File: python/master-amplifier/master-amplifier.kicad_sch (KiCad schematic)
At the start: 8 parts, among them Q1 NPN

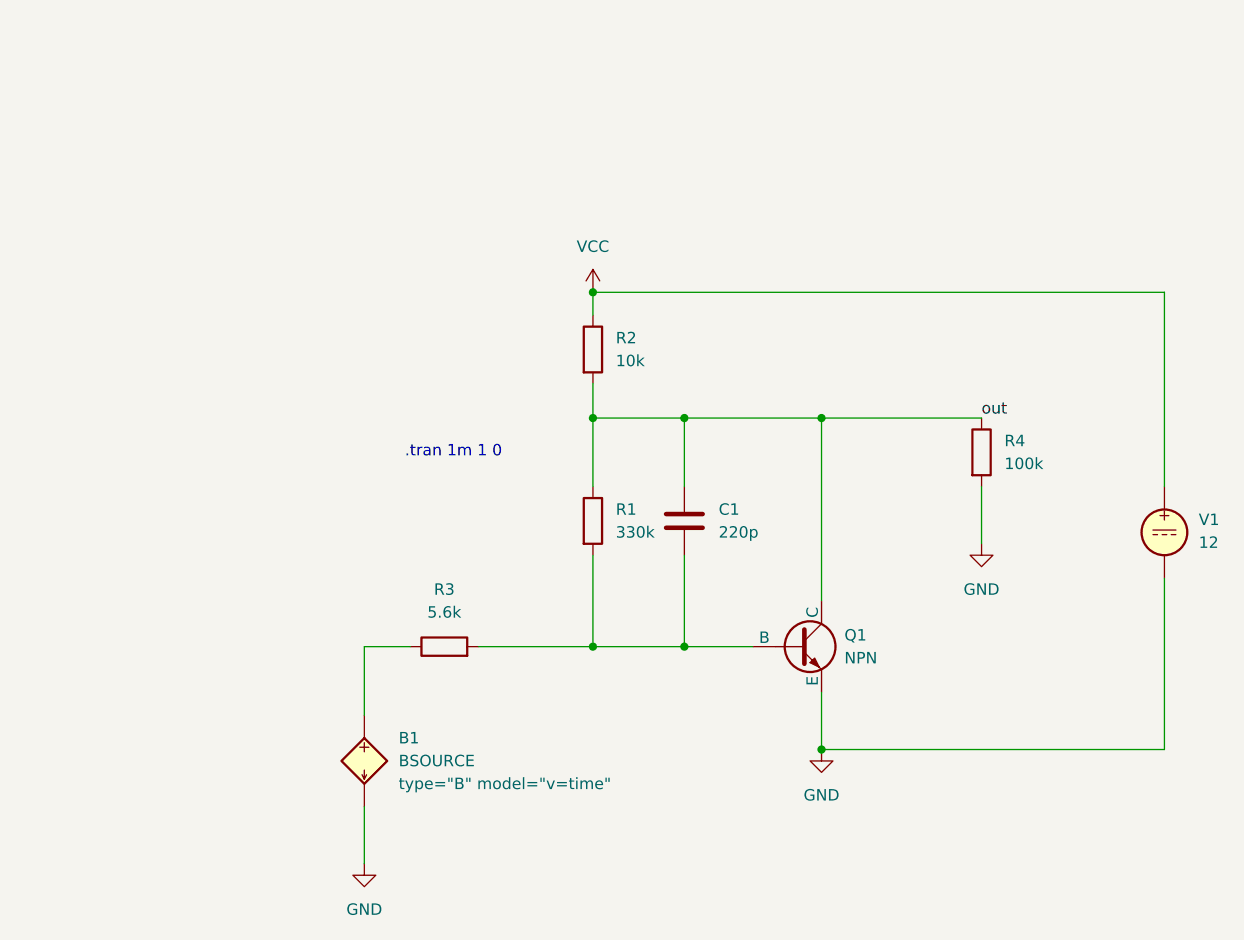
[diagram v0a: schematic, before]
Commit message: something in schematics
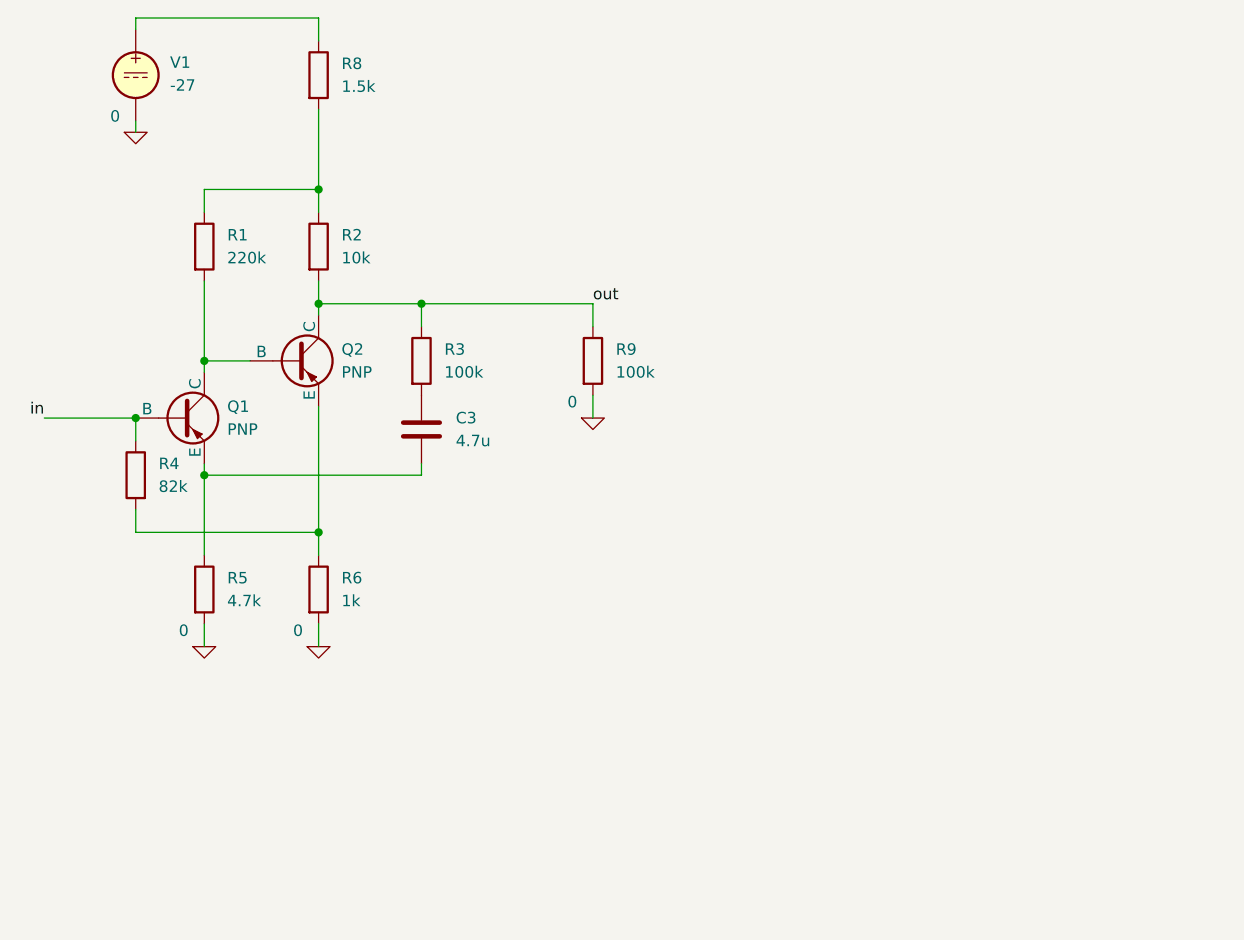
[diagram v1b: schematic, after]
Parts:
- removed B1: BSOURCE, symbol Simulation_SPICE:BSOURCE
- removed C1: 220p, symbol Device:C
- removed Q1: NPN, symbol Simulation_SPICE:NPN
- added C3: 4.7u, symbol Device:C
- added Q1, Q2: PNP, symbol Simulation_SPICE:PNP
- added R5: 4.7k, symbol Device:R
- added R6: 1k, symbol Device:R
- added R8: 1.5k, symbol Device:R
- added R9: 100k, symbol Device:R
- R1: value 330k -> 220k
- R3: value 5.6k -> 100k
- R4: value 100k -> 82k
- V1: value 12 -> -27
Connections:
- net out: now also R3.1, Q2.1 (C), R9.1; no longer R1.1, R4.1
- net at R1.2: now also Q1.1 (C), Q2.2 (B); no longer R3.2
- net GND: no longer names the net of R4.2
- net GND: now also Q2.3 (E), R6.1; no longer V1.2
- net VCC: no longer names the net of R2.1
- net VCC: now also R1.1, R8.2; no longer V1.1
- new net: C3.1, R3.2
- new net: C3.2, Q1.3 (E), R5.1
- new net: R8.1, V1.1
- new net 0: R5.2, R6.2, R9.2, V1.2
- new net in: Q1.2 (B), R4.1
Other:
- note removed: ".tran 1m 1 0"
